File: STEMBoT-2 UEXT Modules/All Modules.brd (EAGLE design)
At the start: 160 x 100 mm, 132 parts, among them IC1 74HC165PW,118, IC2 74HC165PW,118, IC3 74HC165PW,118, J1 FTSH-105-01-XXX-DV-K, J2 FTSH-105-01-XXX-DV-K, J3 FTSH-105-01-XXX-DV-K, J4 FTSH-105-01-XXX-DV-K, J5 FTSH-105-01-XXX-DV-K, J6 FTSH-105-01-XXX-DV-K, Q1 MMBT3904LP-7, Q2 MMBT3904LP-7, Q3 MMBT3904LP-7, U1 TSL260R-LF, U10 SN74HC148D, U11 MAX964ESET, U12 MAX964ESET, U13 HC-SR04(NOSILK), U2 TESEO-LIV3F, U3 CYBLE-012011-00, U4 SN74HC148D, U5 MAX964ESET, U6 MAX964ESET, U7 SN74HC148D, U8 MAX964ESET, U9 MAX964ESET

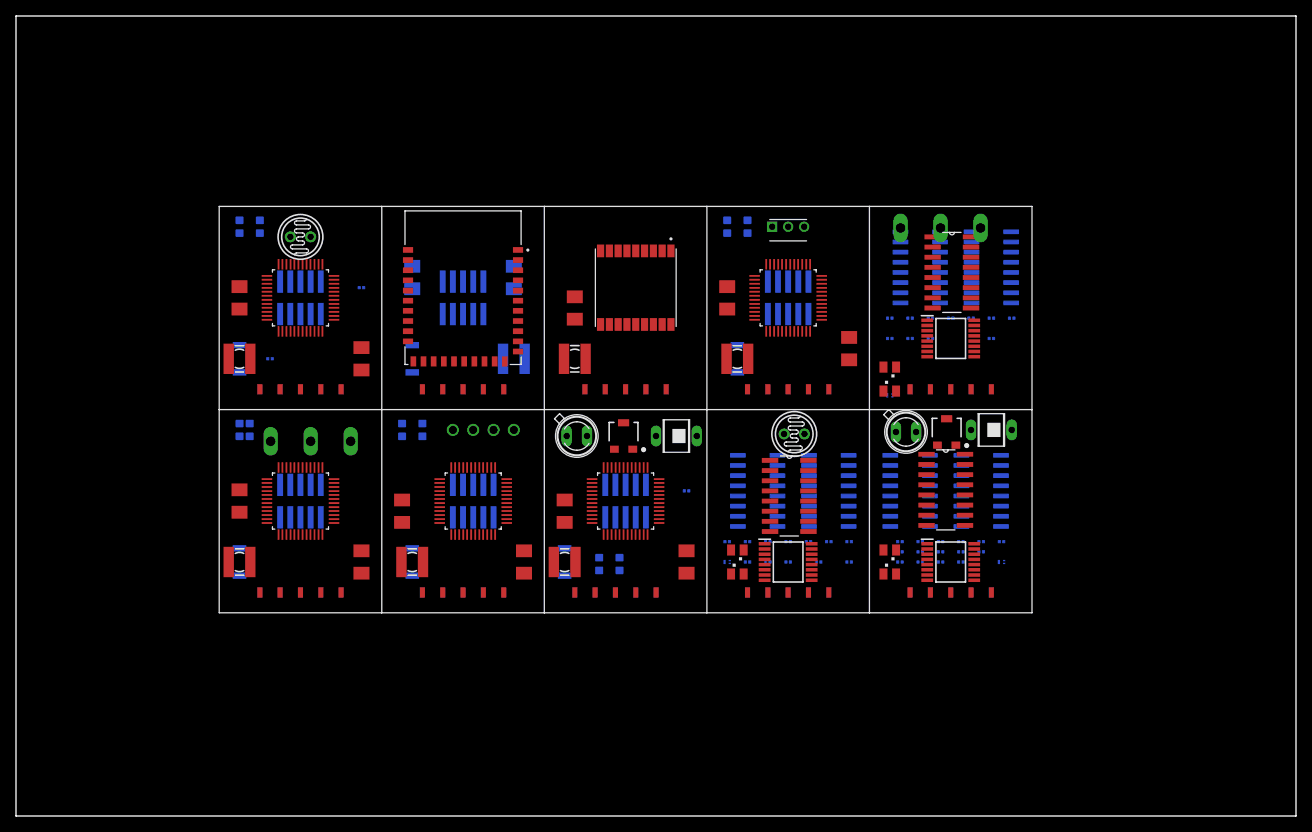
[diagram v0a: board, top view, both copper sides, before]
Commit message: final pcb board layout for reveiw
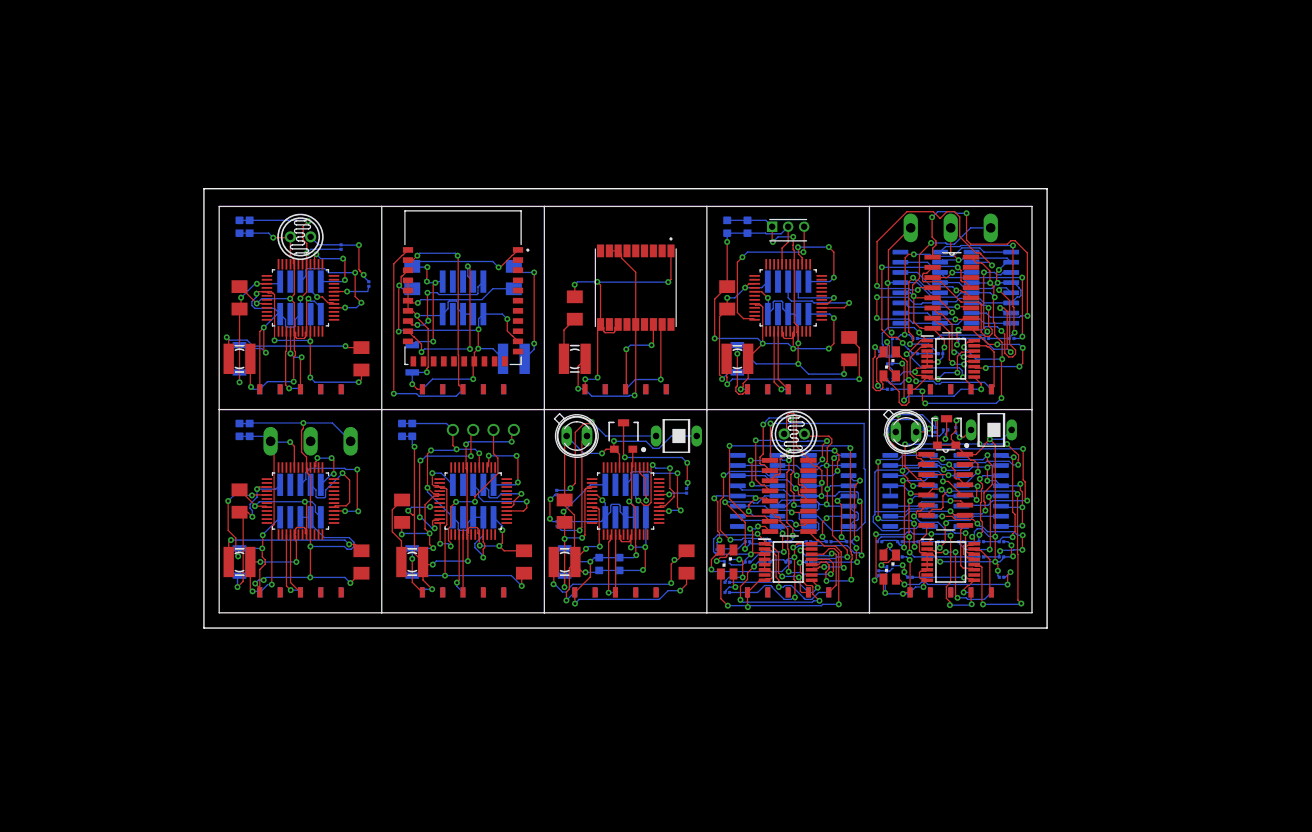
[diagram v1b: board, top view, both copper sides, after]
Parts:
- added R56, R59, R60: ERJ-1RHD3601C, Resistor:RESC0603X26N
- moved R9 17.1 mm to (114.9, 48.3), turned to 270 degrees
- moved R10 17.1 mm to (117.5, 48.3), turned to 270 degrees
- moved R55 16.6 mm to (40.6, 71.1), turned to 270 degrees
- moved R14 14.1 mm to (116.2, 48.3)
- moved Q1 14.0 mm to (109.2, 31.1)
- moved R29 13.0 mm to (124.5, 59.7)
- moved R13 9.94 mm to (111.8, 29.8), turned to 180 degrees
- moved R1 9.53 mm to (112.4, 59.7)
- moved R24 9.25 mm to (115.6, 59.7), turned to 180 degrees
- moved R30 8.89 mm to (109.2, 53.3), turned to 180 degrees
- moved R4 8.03 mm to (88.9, 29.2)
- moved R23 6.35 mm to (88.9, 27.9)
- moved R27 6.29 mm to (112.4, 57.8), turned to 180 degrees
- moved R12 5.43 mm to (123.2, 29.8)
- moved R37 5.12 mm to (120.7, 32.4)
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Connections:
- removed net N$145: IC2.1, U$2.8
- removed net N$159: R61.1
- removed net N$163: IC3.1, U$1.8
- removed net N$2: U1.3
- new net N$158: IC3.1, R56.1, U$1.8
- new net N$164: IC2.1, R60.1, U$2.8
- net N$100: now also U4.13; no longer U4.1
- net N$125: now also U1.3
- net N$157: now also R61.1
- net N$162: now also R59.1
- net N$20: no longer IC1.10
- net N$39: now also IC1.14, IC1.3, IC1.4, IC1.5, IC1.6, R59.2
- net N$43: now also U7.1; no longer U7.13
- net N$44: now also U7.13; no longer U7.1
- net N$53: no longer IC2.10
- net N$55: now also R56.2
- net N$64: now also IC2.14, IC2.3, IC2.4, IC2.5, IC2.6, R60.2
- net N$68: now also U10.1; no longer U10.13
- net N$69: now also U10.13; no longer U10.1
- net N$99: now also U4.1; no longer U4.13
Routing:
- net N$55: track 0.00 -> 118.9 mm, vias 0 -> 20
- net N$144: track 0.00 -> 91.9 mm, vias 0 -> 11
- net N$161: track 0.00 -> 83.5 mm, vias 0 -> 10
- net N$39: track 0.00 -> 78.3 mm, vias 0 -> 10
- net N$108: track 0.00 -> 76.9 mm, vias 0 -> 9
- net N$138: track 0.00 -> 76.6 mm, vias 0 -> 9
- net N$64: track 0.00 -> 75.5 mm, vias 0 -> 9
- net N$79: track 0.00 -> 75.2 mm, vias 0 -> 9
- net N$12: track 0.00 -> 74.7 mm, vias 0 -> 7
- net N$51: track 0.00 -> 73.8 mm, vias 0 -> 7
- net N$109: track 0.00 -> 70.5 mm, vias 0 -> 5
- net N$113: track 0.00 -> 70.5 mm, vias 0 -> 11
- net N$137: track 0.00 -> 69.2 mm, vias 0 -> 8
- net N$119: track 0.00 -> 67.4 mm, vias 0 -> 7
- net N$1: track 0.00 -> 66.2 mm, vias 0 -> 9
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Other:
- board size 160 x 100 mm -> 105.4 x 54.9 mm
- board text added: "Bluetooth Module"
- board text added: "Capstone Team 8"
- board text added: "GPS Module"
- board text added: "Infared Proximity Module"
- board text added: "Infared Remote Module"
- board text added: "Photoresistor Module"
- board text added: "Potentiometer Module"
- board text added: "Ultrasonic Module"
